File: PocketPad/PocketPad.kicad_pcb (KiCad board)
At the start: 2 copper layers, 72.6 x 62.7 mm, 39 parts, among them SW0 SW_Push, SW1 SW_Push, SW10 SW_Push, SW11 SW_Push, SW12 SW_Push, SW13 SW_Push, SW14 SW_Push, SW15 SW_Push, SW16 SW_Push, SW17 SW_Push, SW18 SW_Push, SW2 SW_Push, SW3 SW_Push, SW4 SW_Push, SW5 SW_Push, SW6 SW_Push, SW7 SW_Push, SW8 SW_Push, SW9 SW_Push

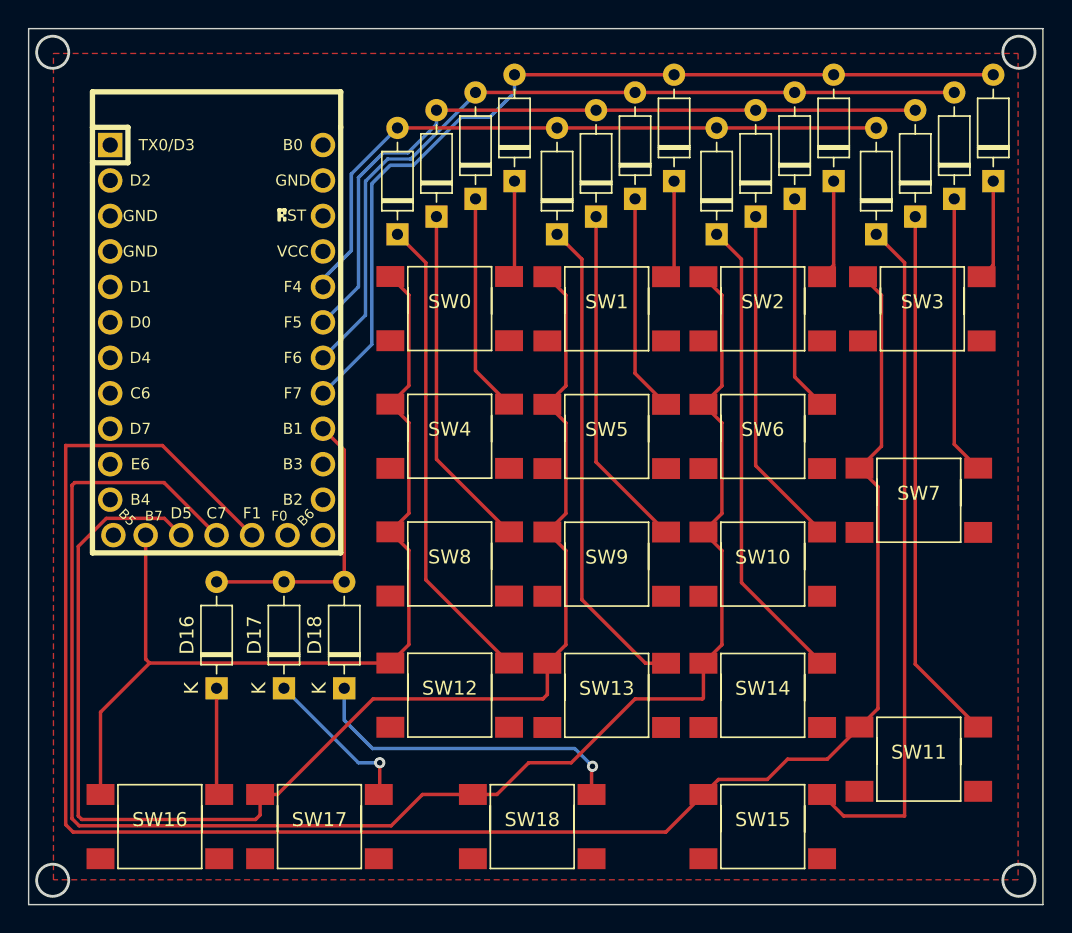
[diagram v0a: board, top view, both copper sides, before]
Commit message: Mounting Holes
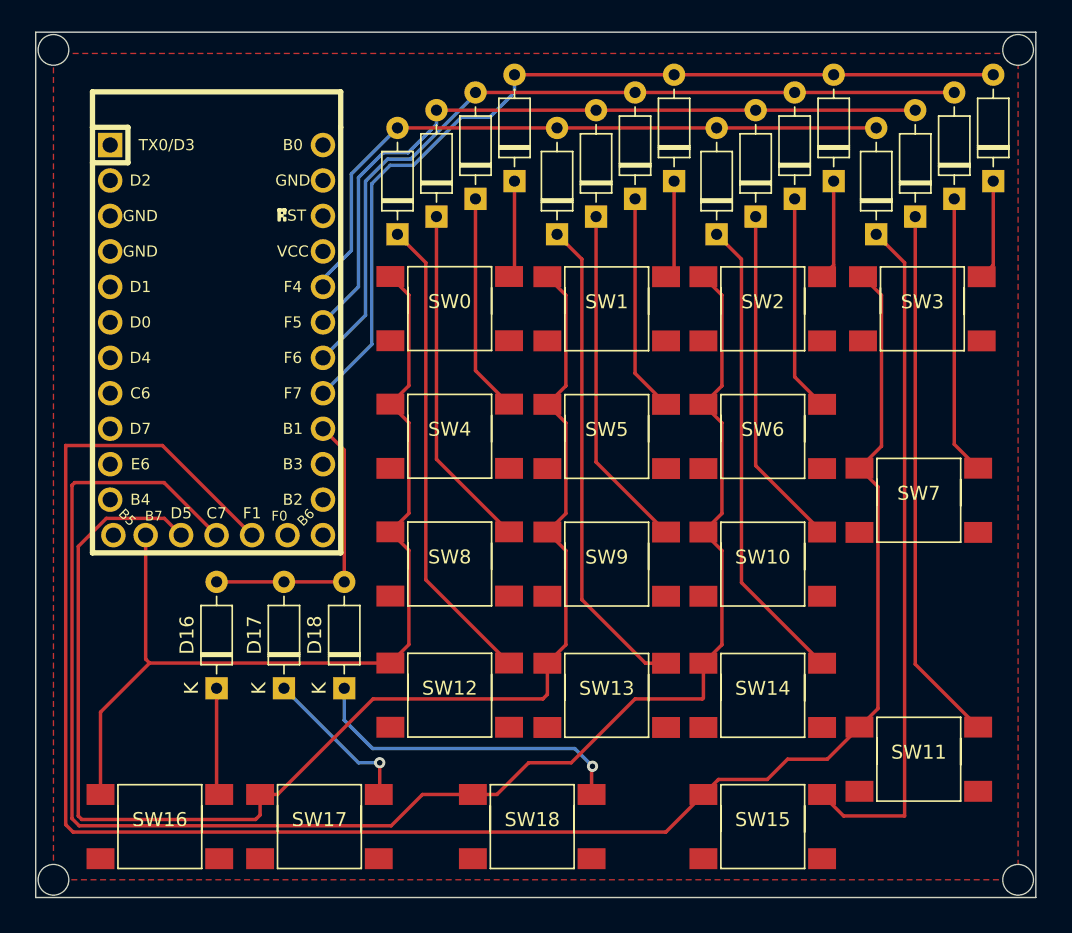
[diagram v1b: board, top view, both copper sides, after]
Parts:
- added REF**: MountingHole_2.2mm_M2, MountingHole:MountingHole_2.2mm_M2, F.Cu at (25.7, 96.3)
- added REF**: MountingHole_2.2mm_M2, MountingHole:MountingHole_2.2mm_M2, F.Cu at (94.7, 36.8)
- added REF**: MountingHole_2.2mm_M2, MountingHole:MountingHole_2.2mm_M2, F.Cu at (25.7, 36.8)
- added REF**: MountingHole_2.2mm_M2, MountingHole:MountingHole_2.2mm_M2, F.Cu at (94.7, 96.3)
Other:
- board size 72.6 x 62.7 mm -> 71.6 x 62 mm
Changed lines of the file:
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@@
     )
+  )
+  (footprint "MountingHole:MountingHole_2.2mm_M2" (layer "F.Cu")
+    (at 25.654 96.266)
+    (descr "Mounting Hole 2.2mm, no annular, M2")
+    (tags "mounting hole 2.2mm no annular m2")
+    (attr exclude_from_pos_files exclude_from_bom)
+    (fp_text reference "REF**" (at 0 -3.2) (layer "F.SilkS") hide
+      (effects (font (size 1 1) (thickness 0.15)))
+    )
+    (fp_text value "MountingHole_2.2mm_M2" (at 0 3.2) (layer "F.Fab") hide
+      (effects (font (size 1 1) (thickness 0.15)))
+    )
+    (fp_text user "${REFERENCE}" (at 0 0) (layer "F.Fab") hide
+      (effects (font (size 1 1) (thickness 0.15)))
+    )
+    (fp_circle (center 0 0) (end 2.2 0) (layer "Cmts.User") (width 0.15) (fill none))
+    (fp_circle (center 0 0) (end 2.45 0) (layer "F.CrtYd") (width 0.05) (fill none))
+    (pad "" np_thru_hole circle (at 0 0) (size 2.2 2.2) (drill 2.2) (layers *.Cu *.Mask))
+  )
+  (footprint "MountingHole:MountingHole_2.2mm_M2" (layer "F.Cu")
+    (at 94.742 36.83)
+    (descr "Mounting Hole 2.2mm, no annular, M2")
+    (tags "mounting hole 2.2mm no annular m2")
+    (attr exclude_from_pos_files exclude_from_bom)
+    (fp_text reference "REF**" (at 0 -3.2) (layer "F.SilkS") hide
+      (effects (font (size 1 1) (thickness 0.15)))
+    )
+    (fp_text value "MountingHole_2.2mm_M2" (at 0 3.2) (layer "F.Fab") hide
+      (effects (font (size 1 1) (thickness 0.15)))
+    )
+    (fp_text user "${REFERENCE}" (at 0 0) (layer "F.Fab") hide
+      (effects (font (size 1 1) (thickness 0.15)))
+    )
+    (fp_circle (center 0 0) (end 2.2 0) (layer "Cmts.User") (width 0.15) (fill none))
+    (fp_circle (center 0 0) (end 2.45 0) (layer "F.CrtYd") (width 0.05) (fill none))
+    (pad "" np_thru_hole circle (at 0 0) (size 2.2 2.2) (drill 2.2) (layers F&B.Cu *.Mask))
   )
   (footprint "Keebio:Switch_6x6x8.5" (layer "F.Cu")
@@
     )
   )
+  (footprint "MountingHole:MountingHole_2.2mm_M2" (layer "F.Cu")
+    (at 25.654 36.83)
+    (descr "Mounting Hole 2.2mm, no annular, M2")
+    (tags "mounting hole 2.2mm no annular m2")
+    (attr exclude_from_pos_files exclude_from_bom)
+    (fp_text reference "REF**" (at 0 -3.2) (layer "F.SilkS") hide
+      (effects (font (size 1 1) (thickness 0.15)))
+    )
+    (fp_text value "MountingHole_2.2mm_M2" (at 0 3.2) (layer "F.Fab") hide
+      (effects (font (size 1 1) (thickness 0.15)))
+    )
+    (fp_text user "${REFERENCE}" (at 0 0) (layer "F.Fab") hide
+      (effects (font (size 1 1) (thickness 0.15)))
+    )
+    (fp_circle (center 0 0) (end 2.2 0) (layer "Cmts.User") (width 0.15) (fill none))
+    (fp_circle (center 0 0) (end 2.45 0) (layer "F.CrtYd") (width 0.05) (fill none))
+    (pad "" np_thru_hole circle (at 0 0) (size 2.2 2.2) (drill 2.2) (layers F&B.Cu *.Mask))
+  )
   (footprint "Diode_THT:D_DO-35_SOD27_P7.62mm_Horizontal" (layer "F.Cu")
     (at 84.582 50.038 90)
@@
     )
   )
+  (footprint "MountingHole:MountingHole_2.2mm_M2" (layer "F.Cu")
+    (at 94.742 96.266)
+    (descr "Mounting Hole 2.2mm, no annular, M2")
+    (tags "mounting hole 2.2mm no annular m2")
+    (attr exclude_from_pos_files exclude_from_bom)
+    (fp_text reference "REF**" (at 0 -3.2) (layer "F.SilkS") hide
+      (effects (font (size 1 1) (thickness 0.15)))
+    )
+    (fp_text value "MountingHole_2.2mm_M2" (at 0 3.2) (layer "F.Fab") hide
+      (effects (font (size 1 1) (thickness 0.15)))
+    )
+    (fp_text user "${REFERENCE}" (at 0 0) (layer "F.Fab") hide
+      (effects (font (size 1 1) (thickness 0.15)))
+    )
+    (fp_circle (center 0 0) (end 2.2 0) (layer "Cmts.User") (width 0.15) (fill none))
+    (fp_circle (center 0 0) (end 2.45 0) (layer "F.CrtYd") (width 0.05) (fill none))
+    (pad "" np_thru_hole circle (at 0 0) (size 2.2 2.2) (drill 2.2) (layers *.Cu *.Mask))
+  )
   (footprint "Keebio:Switch_6x6x8.5" (layer "F.Cu")
     (at 76.454 64.516)
@@
     )
   )
-  (gr_circle (center 94.8 96.3) (end 95.95 96.3) (layer "Edge.Cuts") (width 0.2) (fill none))
-  (gr_circle (center 25.6 96.3) (end 26.75 96.3) (layer "Edge.Cuts") (width 0.2) (fill none))
-  (gr_rect (start 23.876 35.306) (end 96.52 98.044) (layer "Edge.Cuts") (width 0.1) (fill none))
-  (gr_circle (center 25.6 37) (end 26.75 37) (layer "Edge.Cuts") (width 0.2) (fill none))
-  (gr_circle (center 94.8 37) (end 95.95 37) (layer "Edge.Cuts") (width 0.2) (fill none))
+  (gr_rect (start 24.384 35.56) (end 96.012 97.536) (layer "Edge.Cuts") (width 0.1) (fill none))
   (segment (start 49.022 87.884) (end 49.022 90.088) (width 0.25) (layer "F.Cu") (net 3))
   (segment (start 49.022 90.088) (end 48.954 90.156) (width 0.25) (layer "F.Cu") (net 3))
